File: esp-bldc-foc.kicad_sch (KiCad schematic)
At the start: 9 parts, among them J10 UART, J7 A, J8 B, J9 C

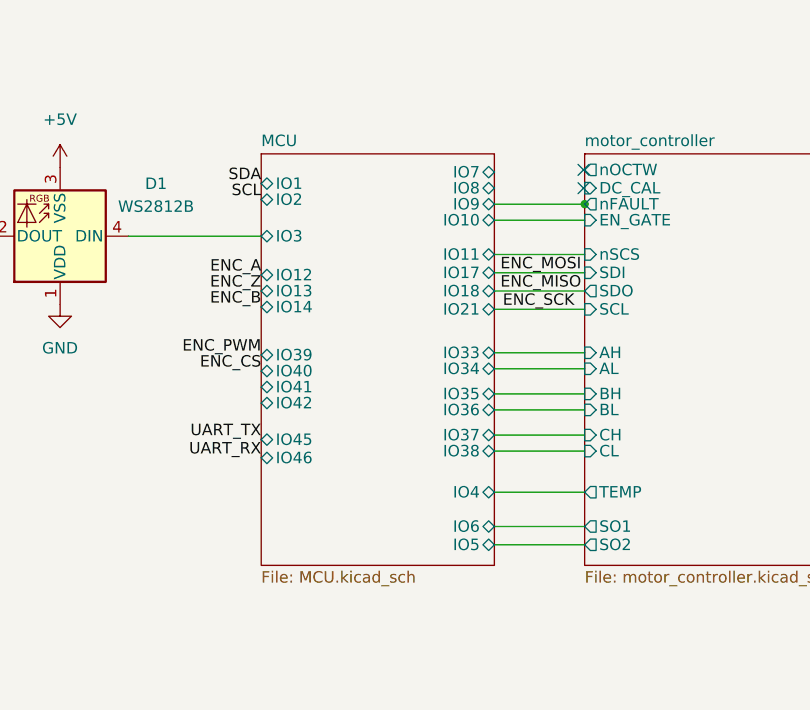
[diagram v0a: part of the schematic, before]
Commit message: Routing done
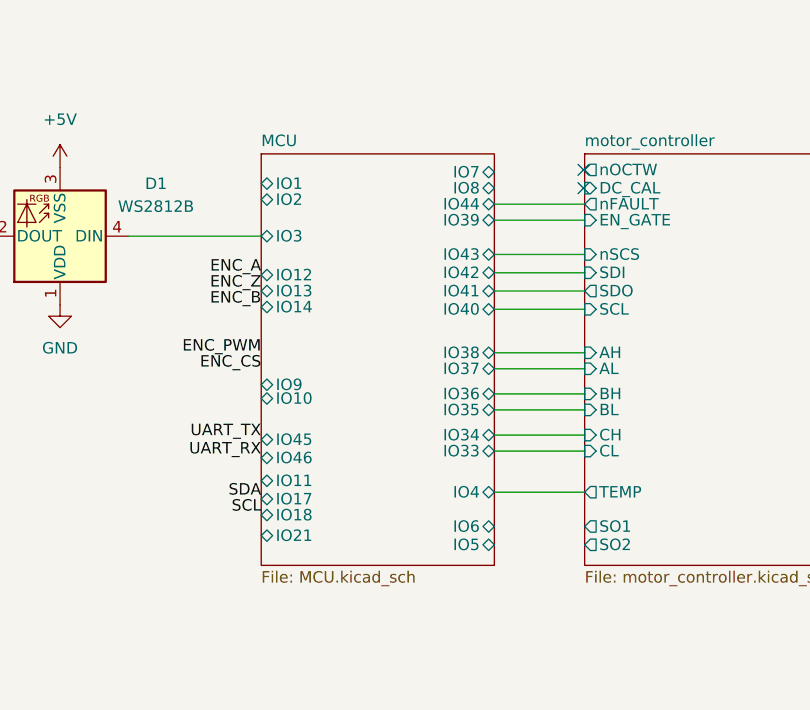
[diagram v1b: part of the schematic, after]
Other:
- sheet MCU ports: added IO43, IO44; removed none
